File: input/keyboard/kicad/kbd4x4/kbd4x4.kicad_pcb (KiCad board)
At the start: 2 copper layers, 80 x 80 mm, 16 parts, among them SW0 mykbd, SW1 mykbd, SW10 mykbd, SW11 mykbd, SW12 mykbd, SW13 mykbd, SW14 mykbd, SW15 mykbd, SW2 mykbd, SW3 mykbd, SW4 mykbd, SW5 mykbd, SW6 mykbd, SW7 mykbd, SW8 mykbd, SW9 mykbd

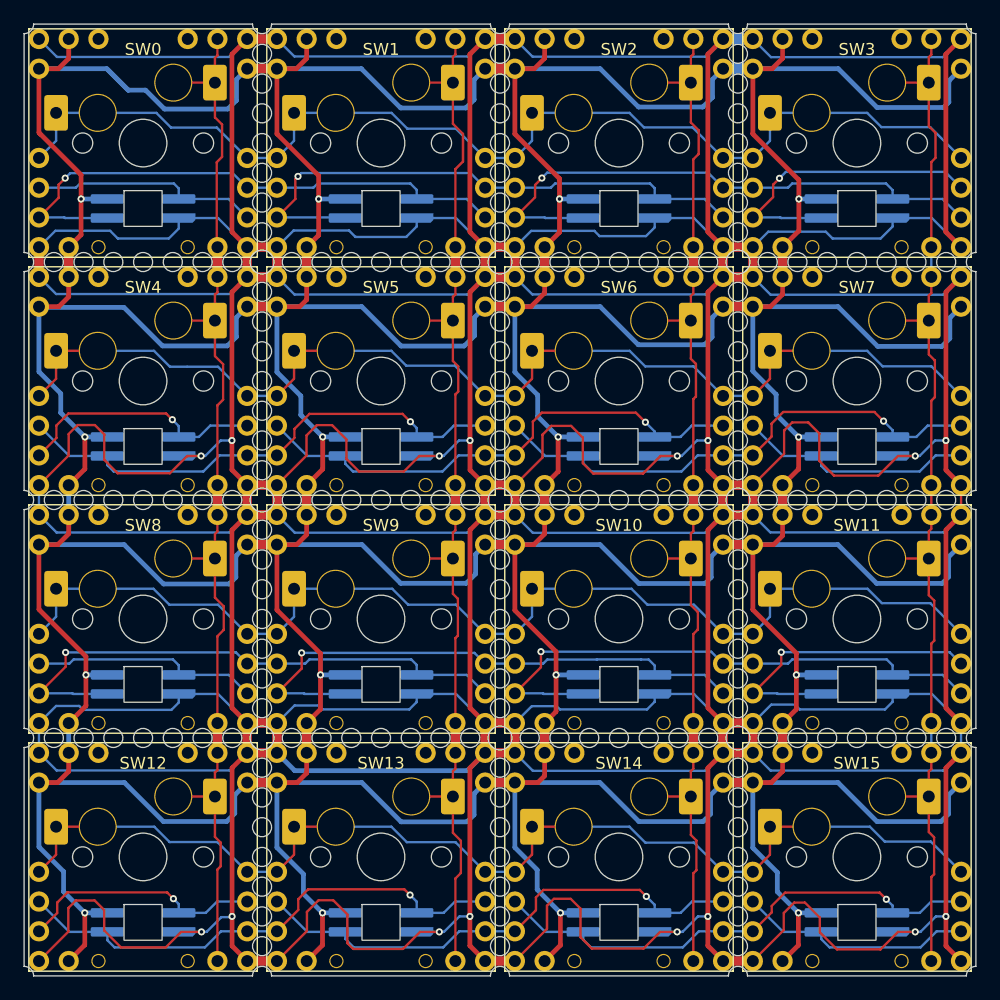
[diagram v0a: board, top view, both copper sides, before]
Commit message: input/keyboard: newest working version
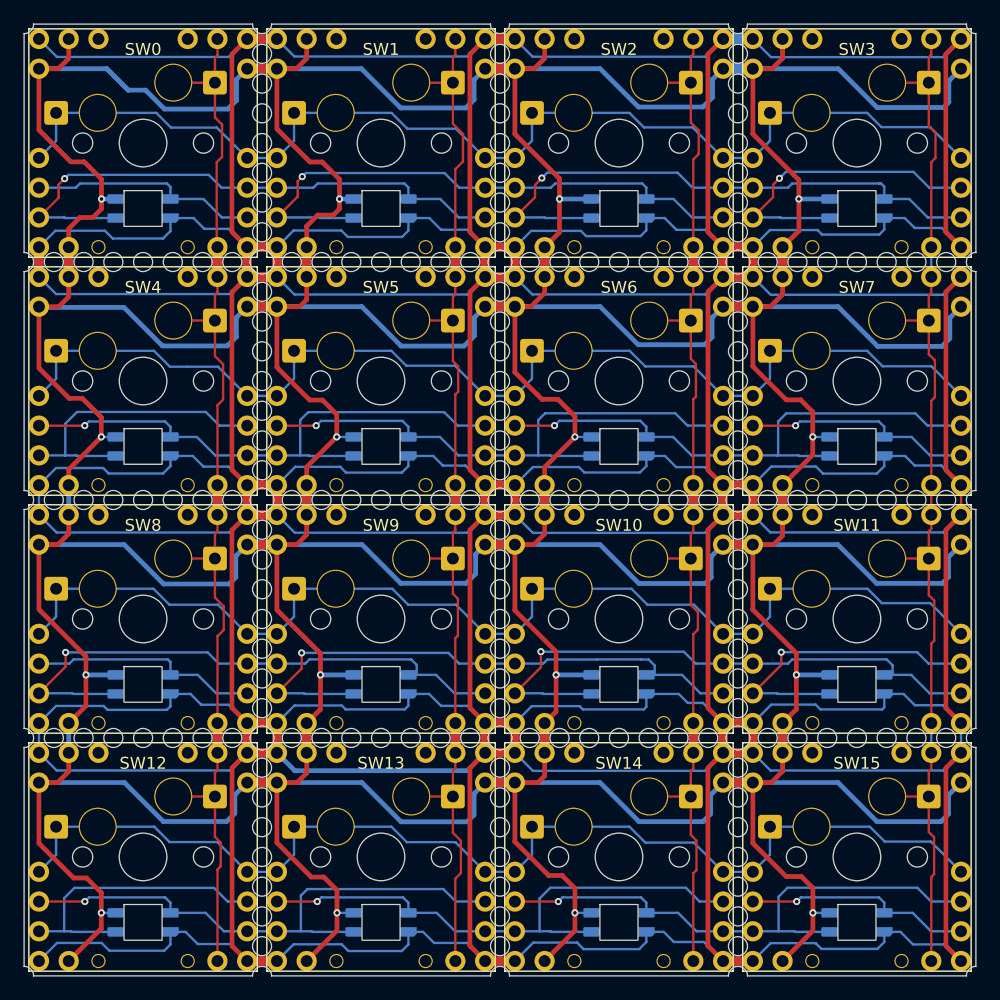
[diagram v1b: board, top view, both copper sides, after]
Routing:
- net GND: track 1080.2 -> 1042.7 mm, vias 16 -> 0
- net VCC: track 778.8 -> 792.9 mm
- net unconnected-(SW12-Pad4): track 20.9 -> 25.5 mm, vias 1 -> 0
- net Net-(SW14-Pad3): track 43.2 -> 47.3 mm
- net unconnected-(SW4-Pad4): track 21.3 -> 25.3 mm, vias 1 -> 0
- net Net-(SW4-Pad3): track 43.6 -> 47.5 mm
- net Net-(SW5-Pad3): track 43.8 -> 47.5 mm
- net Net-(SW13-Pad3): track 43.7 -> 47.3 mm
- net Net-(SW12-Pad3): track 43.8 -> 47.4 mm
- net Net-(SW6-Pad3): track 43.8 -> 47.3 mm
- net Net-(SW2-Pad4): track 47.7 -> 48.6 mm
- net unconnected-(SW7-Pad3): track 20.1 -> 19.3 mm, vias 0 -> 1
- net unconnected-(SW3-Pad4): track 26.0 -> 26.7 mm
- net unconnected-(SW15-Pad3): track 20.0 -> 19.3 mm, vias 0 -> 1
- net Net-(SW0-Pad4): track 47.9 -> 48.4 mm
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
